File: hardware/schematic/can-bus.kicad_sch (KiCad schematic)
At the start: 1 part, among them U7 SN65HVD230

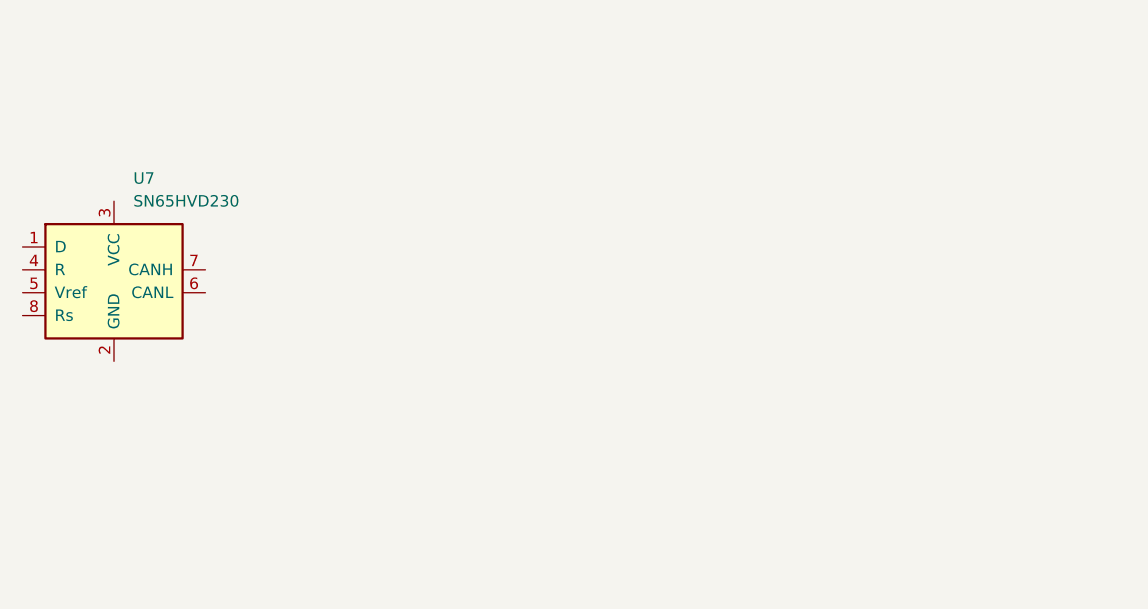
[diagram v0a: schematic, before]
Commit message: schematic finished
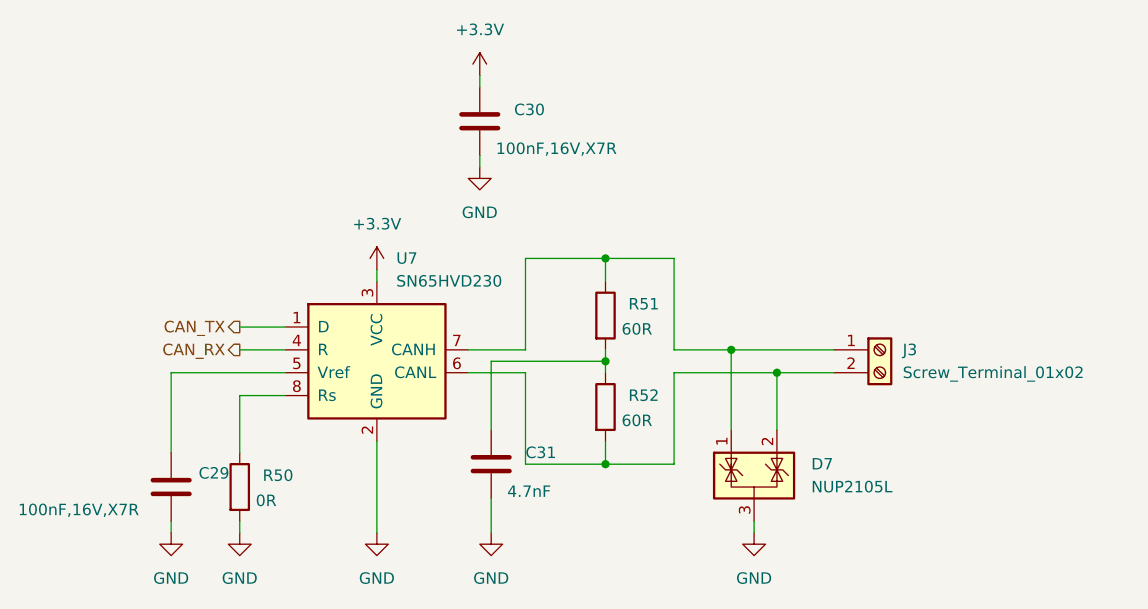
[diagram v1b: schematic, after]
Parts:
- added C29, C30: 100nF,16V,X7R, symbol Device:C
- added C31: 4.7nF, symbol Device:C
- added D7: NUP2105L, Package_TO_SOT_SMD:SOT-23W_Handsoldering, symbol Power_Protection:NUP2105L
- added J3: Screw_Terminal_01x02, TerminalBlock_TE-Connectivity:TerminalBlock_TE_282834-2_1x02_P2.54mm_Horizontal, symbol Connector:Screw_Terminal_01x02
- added R50: 0R, Resistor_SMD:R_0805_2012Metric_Pad1.20x1.40mm_HandSolder, symbol Device:R
- added R51, R52: 60R, Resistor_SMD:R_0805_2012Metric_Pad1.20x1.40mm_HandSolder, symbol Device:R
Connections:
- net CAN_TX: now reaches U7.1 (D)
- net GND: now reaches U7.2 (GND)
- net GND: now also C29.2, C30.2, C31.2, D7.3 (A), R50.2
- net +3.3V: now reaches U7.3 (VCC)
- net +3.3V: now also C30.1
- net CAN_RX: now reaches U7.4 (R)
- net at U7.5 (Vref): now also C29.1
- net at U7.6 (CANL): now also D7.2 (K), J3.2 (Pin_2), R52.2
- net at U7.7 (CANH): now also D7.1 (K), J3.1 (Pin_1), R51.1
- net at U7.8 (Rs): now also R50.1
- new net: C31.1, R51.2, R52.1
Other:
- moved on the sheet: U7
